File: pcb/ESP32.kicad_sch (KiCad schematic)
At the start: 33 parts, among them J7 USB_B_Micro, Q1 MMBT3904, Q2 MMBT3904, Q5 BSS138, SW1 RESET, U5 CP2102N-Axx-xQFN24, U6 ESP32-S3-WROOM-1, U9 AP7361C-33E

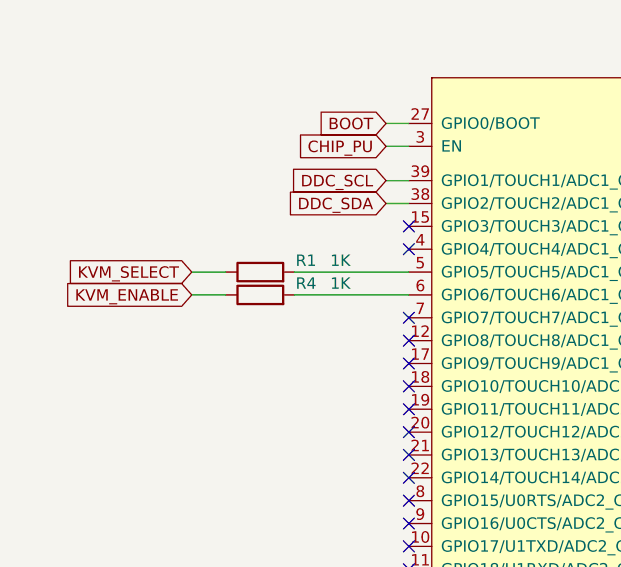
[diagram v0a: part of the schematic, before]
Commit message: routing start
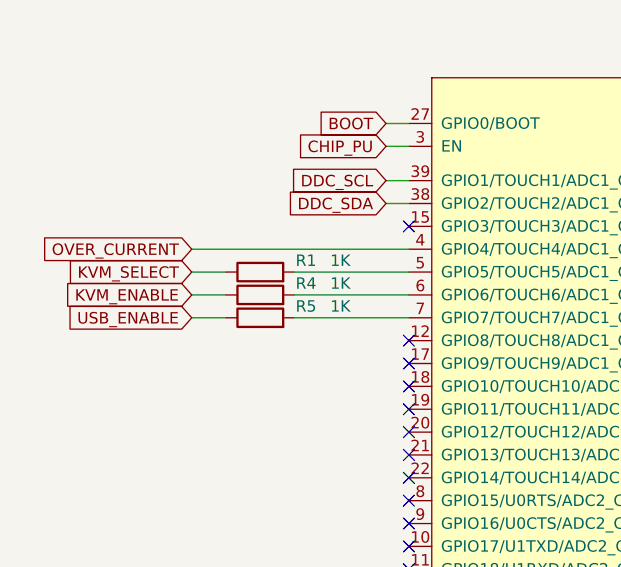
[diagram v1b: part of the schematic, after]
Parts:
- added R5: 1K, Resistor_SMD:R_0603_1608Metric, symbol Device:R
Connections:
- net OVER_CURRENT: now reaches U6.4 (GPIO4/TOUCH4/ADC1_CH3)
- net at U6.7 (GPIO7/TOUCH7/ADC1_CH6): now also R5.2
- new net USB_ENABLE: R5.1
- no-connect marks 39 -> 37
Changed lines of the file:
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@@
   (no_connect (at 106.68 166.37))
   (no_connect (at 172.72 83.82))
-  (no_connect (at 54.61 54.61))
   (no_connect (at 26.67 168.91))
   (no_connect (at 172.72 58.42))
@@
   (no_connect (at 106.68 163.83))
   (no_connect (at 106.68 176.53))
-  (no_connect (at 54.61 62.23))
   (no_connect (at 172.72 73.66))
   (wire (pts (xy 30.48 57.15) (xy 34.29 57.15))
@@
     (stroke (width 0) (type default) (color 0 0 0 0))
   )
+  (wire (pts (xy 41.91 62.23) (xy 54.61 62.23))
+    (stroke (width 0) (type default) (color 0 0 0 0))
+  )
   (wire (pts (xy 93.98 191.77) (xy 93.98 194.31))
     (stroke (width 0) (type default) (color 0 0 0 0))
@@
     (stroke (width 0) (type default) (color 0 0 0 0))
   )
+  (wire (pts (xy 30.48 54.61) (xy 54.61 54.61))
+    (stroke (width 0) (type default) (color 0 0 0 0))
+  )
   (wire (pts (xy 257.81 153.67) (xy 255.27 153.67))
     (stroke (width 0) (type default) (color 0 0 0 0))
@@
     (stroke (width 0) (type default) (color 0 0 0 0))
   )
+  (wire (pts (xy 30.48 62.23) (xy 34.29 62.23))
+    (stroke (width 0) (type default) (color 0 0 0 0))
+  )
   (wire (pts (xy 132.08 153.67) (xy 132.08 157.48))
     (stroke (width 0) (type default) (color 0 0 0 0))
@@
     (stroke (width 0) (type default) (color 0 0 0 0))
   )
+  (global_label "OVER_CURRENT" (shape input) (at 30.48 54.61 180) (fields_autoplaced)
+    (effects (font (size 1.27 1.27)) (justify right))
+    (property "Intersheet References" "${INTERSHEET_REFS}" (id 0) (at 13.6736 54.5306 0)
+      (effects (font (size 1.27 1.27)) (justify right) hide)
+    )
+  )
   (global_label "U0_TXD" (shape input) (at 109.22 143.51 0) (fields_autoplaced)
     (effects (font (size 1.27 1.27)) (justify left))
@@
     (property "Intersheet References" "${INTERSHEET_REFS}" (id 0) (at 256.4606 28.2483 90)
       (effects (font (size 1.27 1.27)) (justify left) hide)
+    )
+  )
+  (global_label "USB_ENABLE" (shape input) (at 30.48 62.23 180) (fields_autoplaced)
+    (effects (font (size 1.27 1.27)) (justify right))
+    (property "Intersheet References" "${INTERSHEET_REFS}" (id 0) (at 16.274 62.1506 0)
+      (effects (font (size 1.27 1.27)) (justify right) hide)
     )
   )
@@
     (pin "4")
   )
+  (symbol (lib_id "Device:R") (at 38.1 62.23 90) (unit 1)
+    (in_bom yes) (on_board yes)
+    (property "Reference" "R5" (id 0) (at 43.18 60.96 90))
+    (property "Value" "1K" (id 1) (at 46.99 60.96 90))
+    (property "Footprint" "Resistor_SMD:R_0603_1608Metric" (id 2) (at 38.1 64.008 90)
+      (effects (font (size 1.27 1.27)) hide)
+    )
+    (property "Datasheet" "~" (id 3) (at 38.1 62.23 0)
+      (effects (font (size 1.27 1.27)) hide)
+    )
+    (pin "1")
+    (pin "2")
+  )
   (symbol (lib_id "power:GND") (at 49.53 175.26 0) (unit 1)
